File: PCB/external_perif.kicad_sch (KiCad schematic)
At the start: 15 parts, among them J1 Bus_ISA_8bit, P1 USB_C_Plug_USB2.0, SW3 SW_Push_Dual, SW4 SW_Push_Dual, U11 CH552T, U5 ESP-12F, U7 RP2354B

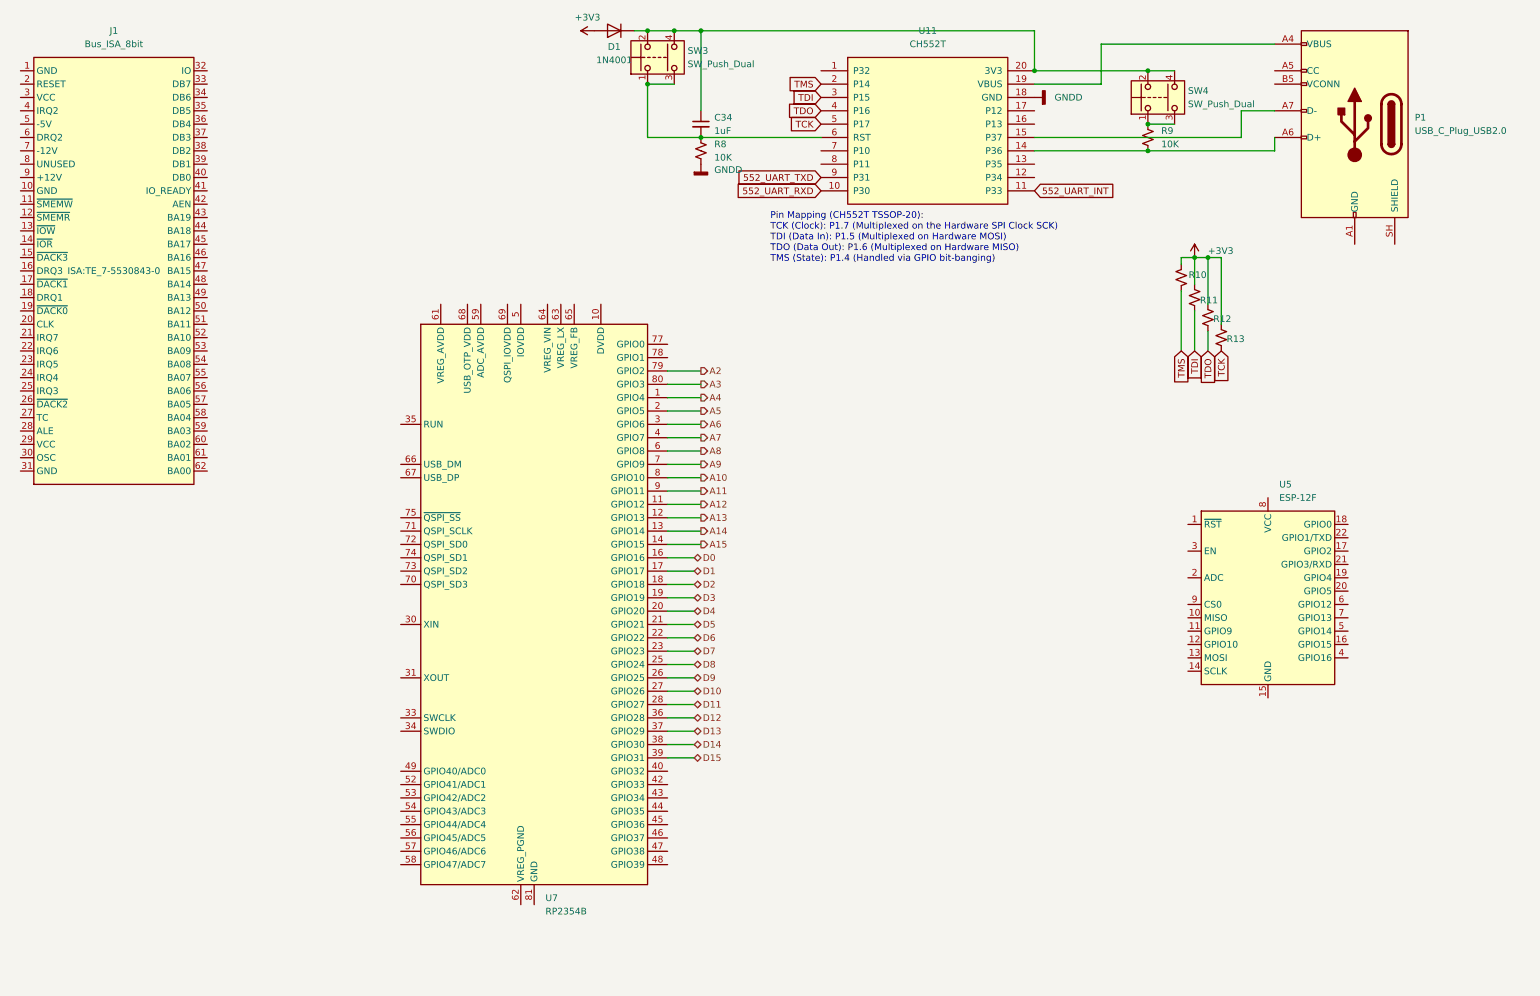
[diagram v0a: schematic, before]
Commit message: route-out in progress
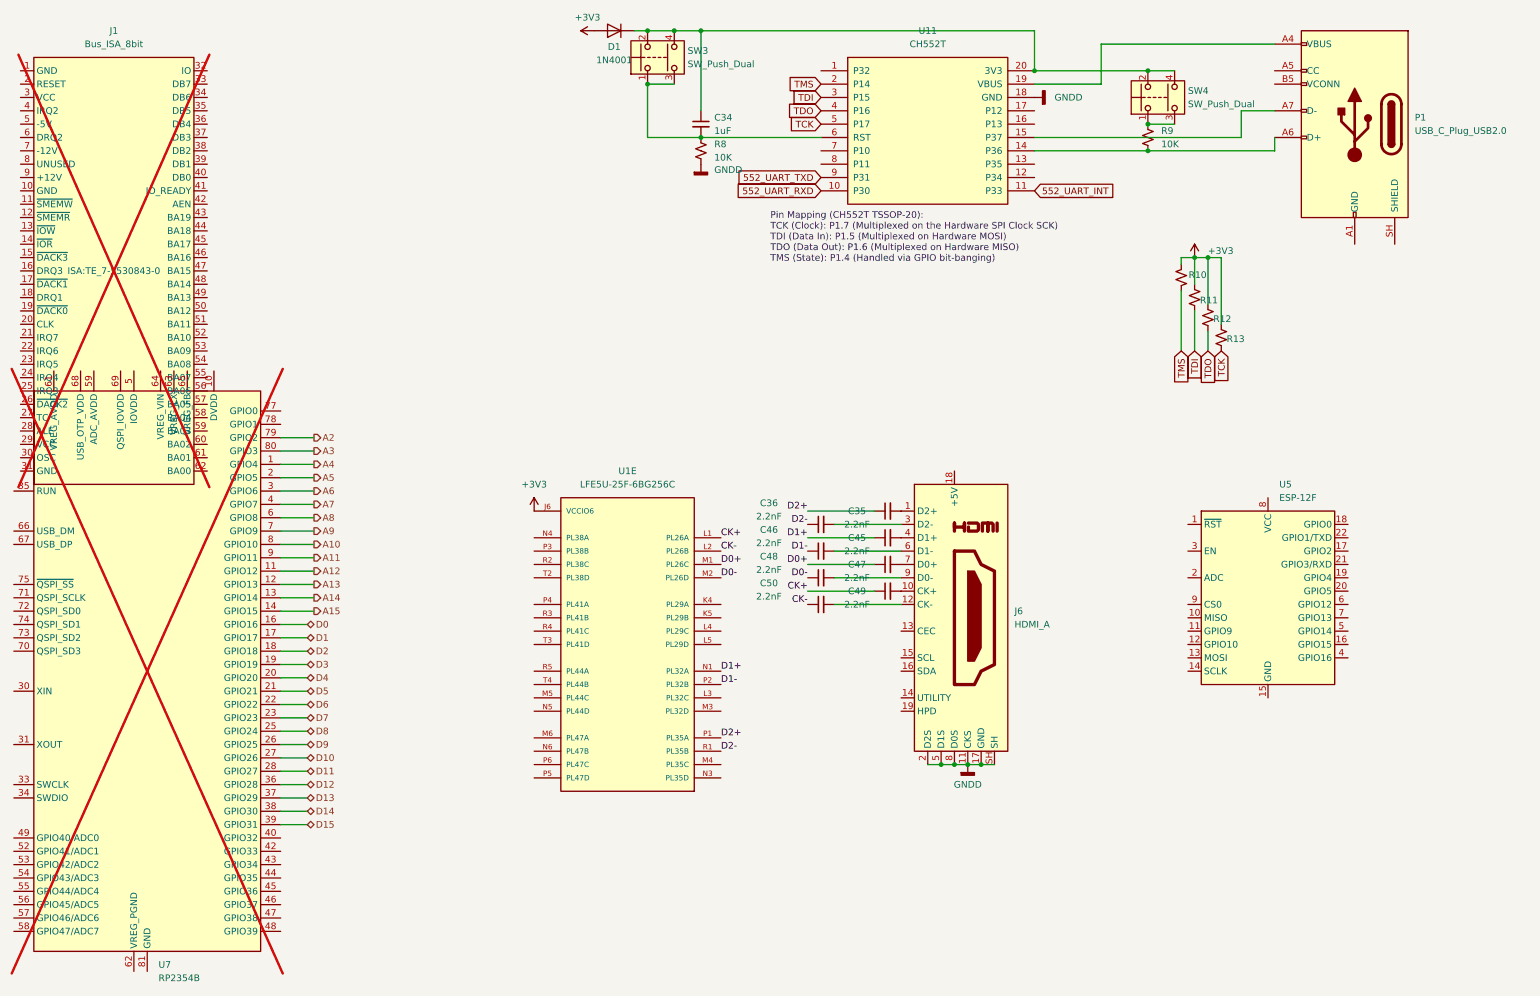
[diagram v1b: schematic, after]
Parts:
- added C35, C36, C45, C46, C47, C48, C49, C50: 2.2nF, Capacitor_SMD:C_01005_0402Metric, symbol Device:C_Small
- added J6: HDMI_A, Connector_Video:HDMI_A_Amphenol_10029449-x01xLF_Horizontal, symbol Connector:HDMI_A
- added U1: LFE5U-25F-6BG256C, ECP5:BGA256C80P16X16_1400X1400X170, symbol Lattice:LFE5U-25F-6BG256C
- J1: now not fitted; now left out of the parts list
- P1: footprint (none) -> Connector_USB:USB_C_Receptacle_GCT_USB4105-xx-A_16P_TopMnt_Horizontal
- SW3, SW4: footprint (none) -> Button_Switch_THT:SW_PUSH_6mm
- U7: private KLC_S4.2_VREG_LX -> (none); now not fitted; now left out of the parts list
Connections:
- net +3V3: now also U1.J6 (VCCIO6), U1.J7 (VCCIO6)
- net GNDD: now also J6.11 (CKS), J6.17 (GND), J6.2 (D2S), J6.5 (D1S), J6.8 (D0S), J6.SH
- new net: C35.2, J6.1 (D2+)
- new net: C49.2, J6.10 (CK+)
- new net: C50.2, J6.12 (CK-)
- new net: C36.2, J6.3 (D2-)
- new net: C45.2, J6.4 (D1+)
- new net: C46.2, J6.6 (D1-)
- new net: C47.2, J6.7 (D0+)
- new net: C48.2, J6.9 (D0-)
- new net CK+: C49.1, U1.L1 (PL26A)
- new net CK-: C50.1, U1.L2 (PL26B)
- new net D0+: C47.1, U1.M1 (PL26C)
- new net D0-: C48.1, U1.M2 (PL26D)
- new net D1+: C45.1, U1.N1 (PL32A)
- new net D1-: C46.1, U1.P2 (PL32B)
- new net D2+: C35.1, U1.P1 (PL35A)
- new net D2-: C36.1, U1.R1 (PL35B)
